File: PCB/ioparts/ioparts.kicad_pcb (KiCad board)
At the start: 2 copper layers, 13 x 8 mm, 13 parts, among them J1 USB_B_Micro, J2 USB_C_Receptacle_USB2.0, J3 Conn_01x04, J4 Conn_01x04, J5 AudioJack4, J6 AudioJack4, J7 Conn_01x04, J8 Conn_01x04

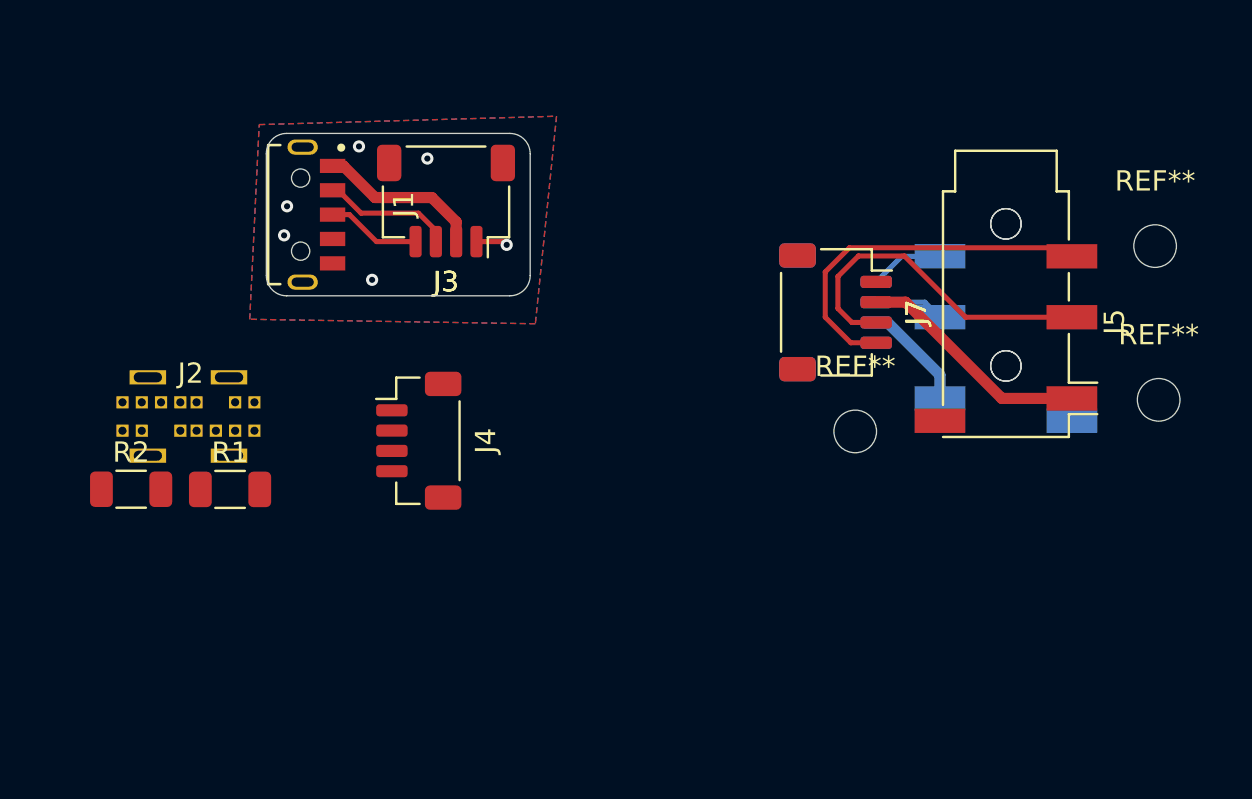
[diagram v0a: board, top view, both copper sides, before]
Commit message: temp
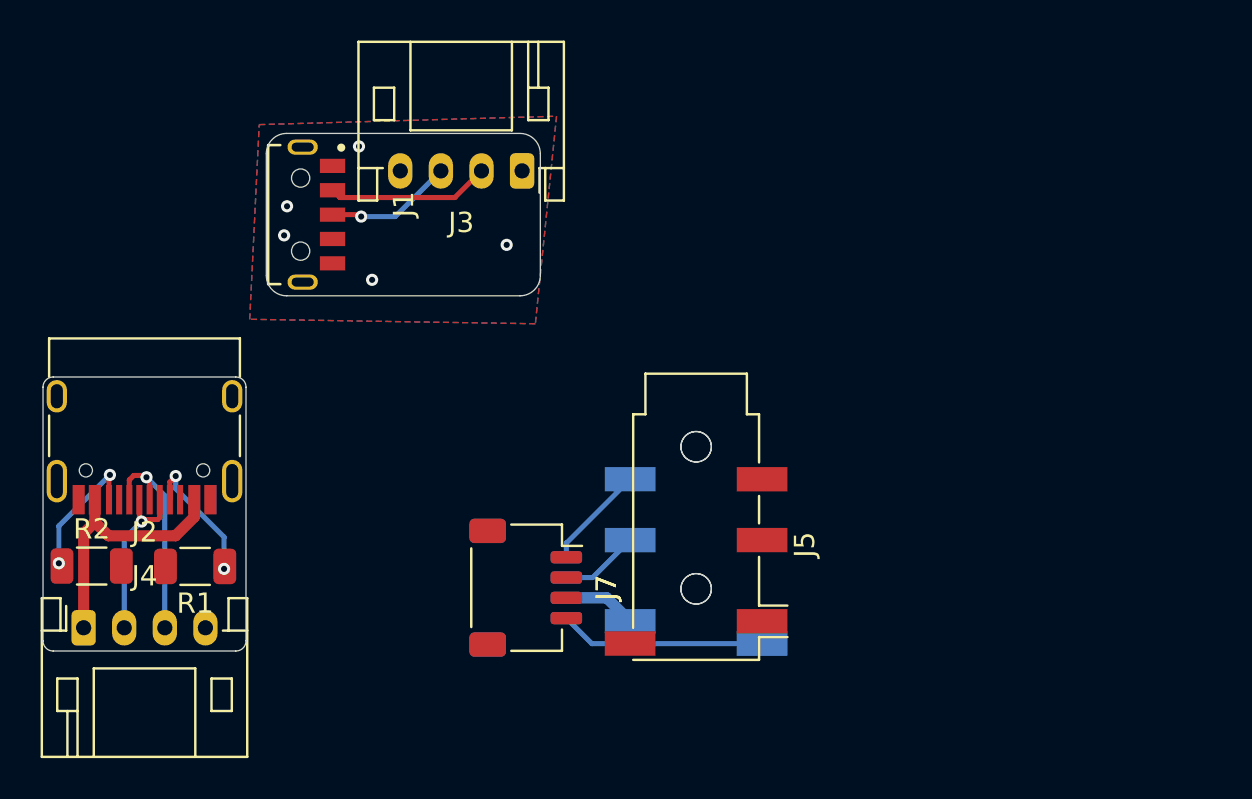
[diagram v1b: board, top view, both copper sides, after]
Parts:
- removed REF** (x3): MountingHole_2.1mm, MountingHole:MountingHole_2.1mm
- J2: footprint ioparts:KH-TYPE-C-L10-14P -> Connector_USB:USB_C_Receptacle_HRO_TYPE-C-31-M-12
- J3: footprint Connector_JST:JST_SH_SM04B-SRSS-TB_1x04-1MP_P1.00mm_Horizontal -> Connector_JST:JST_PH_S4B-PH-K_1x04_P2.00mm_Horizontal
- J4: footprint Connector_JST:JST_SH_BM04B-SRSS-TB_1x04-1MP_P1.00mm_Vertical -> Connector_JST:JST_PH_S4B-PH-K_1x04_P2.00mm_Horizontal
- moved J7 20.4 mm to (118.8, 68.4)
- moved J8 20.4 mm to (118.8, 68.4)
- moved J4 18.9 mm to (97.0, 70.4), turned to 0 degrees
- moved J5 18.8 mm to (127.2, 66.2)
- moved J6 18.8 mm to (127.2, 66.2)
- moved R2 4.25 mm to (97.4, 67.3)
- moved R1 4.17 mm to (102.5, 67.3), turned to 180 degrees
- moved J3 4.03 mm to (118.6, 47.8)
- moved J2 2.16 mm to (100.0, 60.0), turned to 180 degrees
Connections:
- J3 pad 1: GND1 -> VBUS_MICRO
- J3 pad 2: VBUS_MICRO -> DM_MICRO
- J3 pad 3: DM_MICRO -> DP_MICRO
- J3 pad 4: DP_MICRO -> GND1
- J4 pad 1: GND -> VBUS_C
- J4 pad 2: VBUS_C -> DM_C
- J4 pad 3: DM_C -> DP_C
- J4 pad 4: DP_C -> GND
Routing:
- net SDA: track 18.1 -> 0.00 mm
- net SCL: track 16.9 -> 0.00 mm
- net VBUS_C: track 0.00 -> 13.0 mm
- net VBUS_TRRS: track 11.6 -> 0.00 mm
- net DP_C: track 0.00 -> 10.9 mm, vias 0 -> 1
- net GND2: track 0.34 -> 10.2 mm
- net DM_C: track 0.00 -> 8.56 mm, vias 0 -> 1
- net VBUS_MICRO: track 8.20 -> 0.00 mm
- net Net-(J2-PadA5): track 0.00 -> 6.84 mm, vias 0 -> 2
- net Net-(J2-PadB5): track 0.00 -> 6.64 mm, vias 0 -> 2
- net DM_MICRO: track 5.64 -> 8.03 mm
- net VBUS_TRRS_B: track 5.37 -> 3.62 mm
- net DP_MICRO: track 4.64 -> 6.31 mm, vias 0 -> 1
- net GND1: track 1.56 -> 0.00 mm, vias 6 -> 5
- net SDA_B: track 3.66 -> 5.15 mm
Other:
- board size 13 x 8 mm -> 24.5 x 25.5 mm
